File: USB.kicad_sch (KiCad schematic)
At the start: 31 parts, among them J5 USB_C_Receptacle, J6 USB_C_Receptacle, SW1 SW_DIP_x04, U10 TPS2552, U11 TPD4EUSB30, U12 TPD4EUSB30, U13 TPD4EUSB30, U14 TPD4EUSB30, U15 TS3USB221, U16 HD3SS3220, U17 TS3USB221

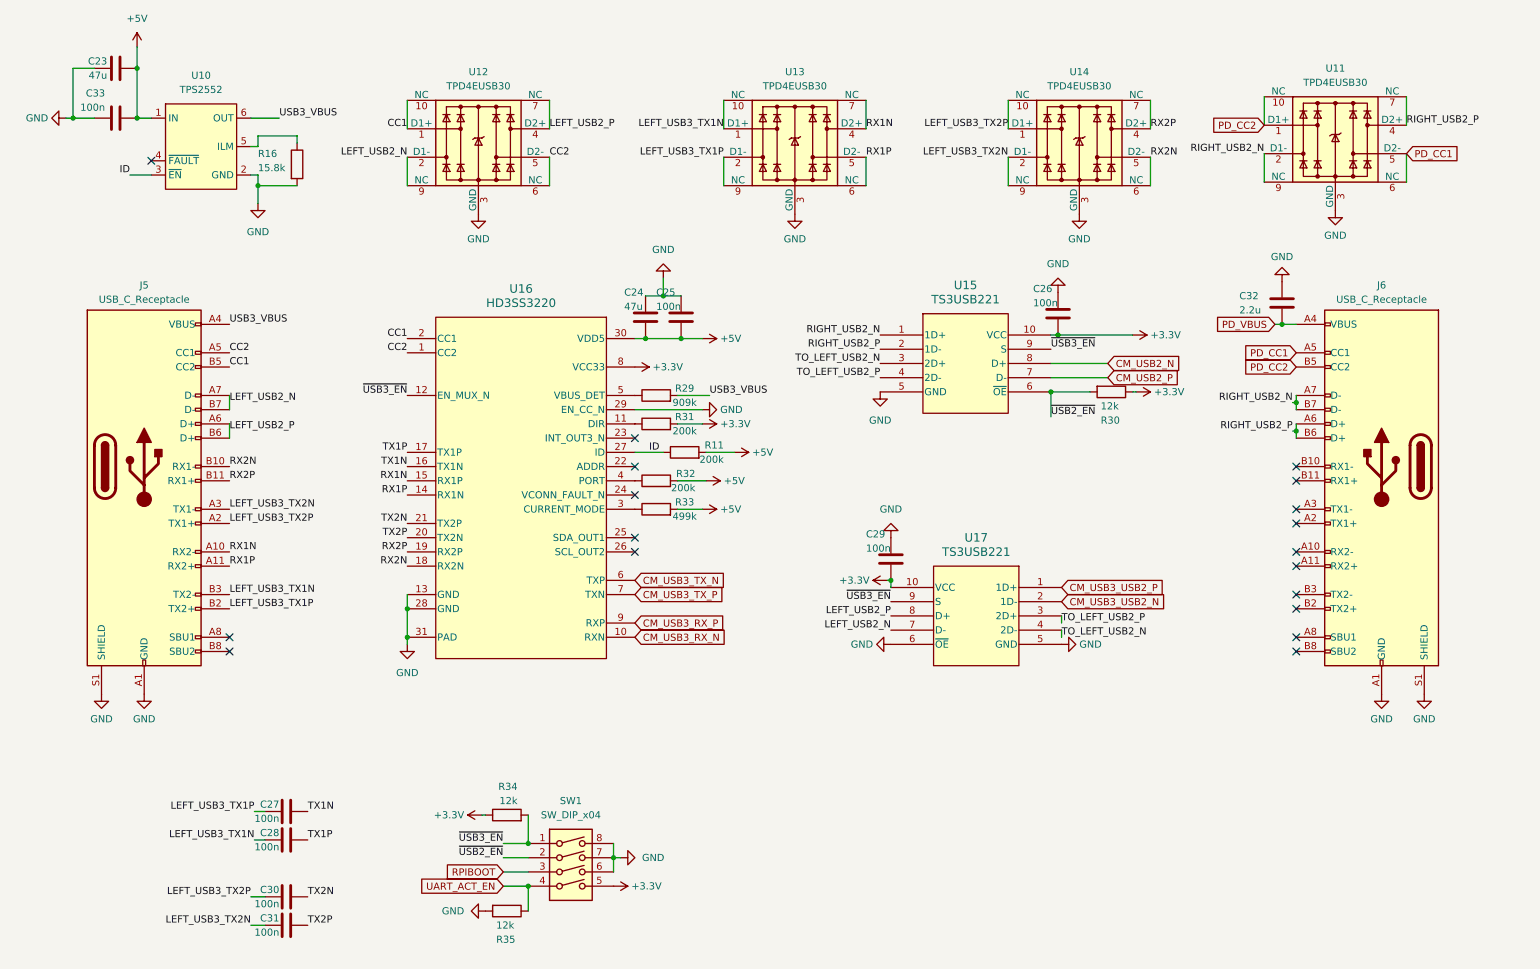
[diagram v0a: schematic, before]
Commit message: wip
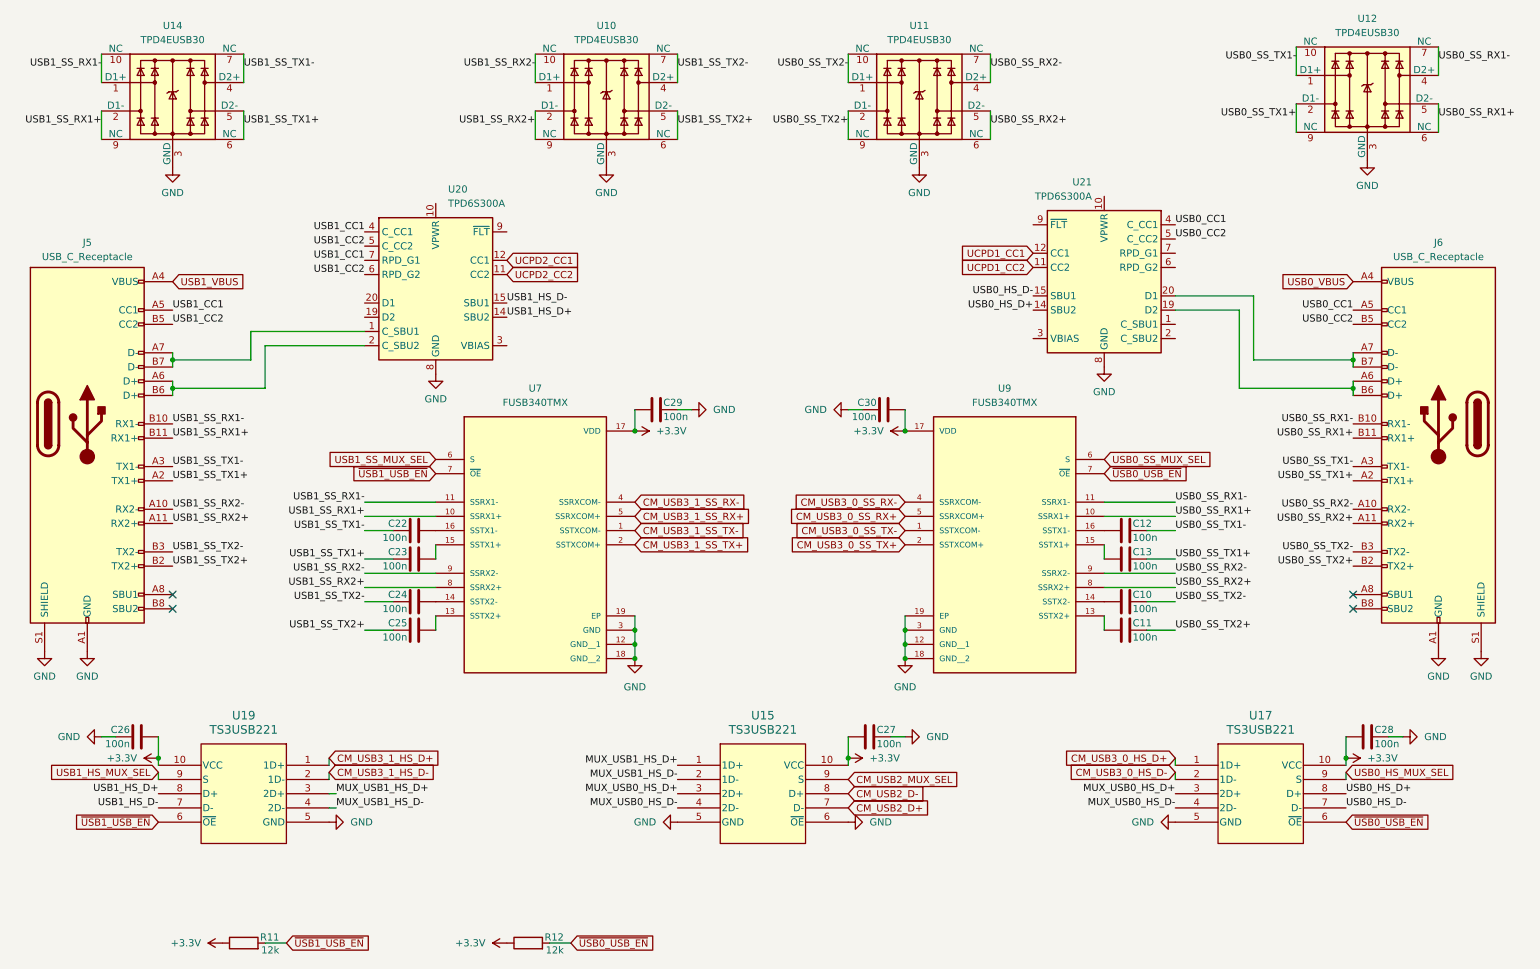
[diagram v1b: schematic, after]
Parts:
- removed C31, C33: 100n, Capacitor_SMD:C_0402_1005Metric, symbol Device:C
- removed C32: 2.2u, Capacitor_SMD:C_1206_3216Metric, symbol Device:C
- removed R16: 15.8k, Resistor_SMD:R_0402_1005Metric, symbol Device:R
- removed R29: 909k, Resistor_SMD:R_0402_1005Metric, symbol Device:R
- removed R30, R34, R35: 12k, Resistor_SMD:R_0402_1005Metric, symbol Device:R
- removed R31, R32: 200k, Resistor_SMD:R_0402_1005Metric, symbol Device:R
- removed R33: 499k, Resistor_SMD:R_0402_1005Metric, symbol Device:R
- removed SW1: SW_DIP_x04, PiCard:SW-SMD_8P-P1.27_EU-04KS, symbol Switch:SW_DIP_x04
- removed U10: TPS2552, Package_TO_SOT_SMD:SOT-23-6, symbol PiCard:TPS2552
- removed U13: TPD4EUSB30, Package_SON:USON-10_2.5x1.0mm_P0.5mm, symbol Power_Protection:TPD4EUSB30
- removed U16: HD3SS3220, PiCard:RNH0030A, symbol PiCard:HD3SS3220
- added C10, C11, C12, C13, C22: 100n, Capacitor_SMD:C_0402_1005Metric, symbol Device:C
- added R12: 12k, Resistor_SMD:R_0402_1005Metric, symbol Device:R
- added U10: TPD4EUSB30, Package_SON:USON-10_2.5x1.0mm_P0.5mm, symbol Power_Protection:TPD4EUSB30
- added U19: TS3USB221, PiCard:RSE10, symbol PiCard:TS3USB221
- added U20, U21: TPD6S300A, Package_DFN_QFN:WQFN-20-1EP_3x3mm_P0.4mm_EP1.7x1.7mm_ThermalVias, symbol Power_Protection:TPD6S300A
- added U7, U9: FUSB340TMX, PiCard:QFN-18-1EP_2x2.8mm_P0.4mm_EP1.05x1.85mm, symbol PiCard:FUSB340TMX
- C23, C24: value 47u -> 100n; footprint Capacitor_SMD:C_0805_2012Metric -> Capacitor_SMD:C_0402_1005Metric; LCSC C16780 -> C307331; MPN CL21A476MQYNNNE -> CL05B104KB54PNC
- R11: value 200k -> 12k; LCSC C25764 -> C25752; MPN 0402WGF2003TCE -> 0402WGF1202TCE
- U15, U17: footprint Package_DFN_QFN:Texas_UQFN-10_1.5x2mm_P0.5mm -> PiCard:RSE10; LCSC C130085 -> (none); MPN TS3USB221RSER -> (none); Manufacturer Texas Instruments -> (none)
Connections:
- net ID is gone; now on net +3.3V: R11.1
- net TX1N is gone; now on net +3.3V: C27.2
- net TX1P is gone; now on net +3.3V: C28.2
- net TX2N is gone; now on net +3.3V: C30.2
- net ~{USB2_EN} is gone; now on net GND: U15.6 (~{OE})
- net +3.3V: now also R12.1, U19.10 (VCC), U7.17 (VDD), U9.17 (VDD)
- net GND: now also C27.1, C28.1, C30.1, U10.3 (GND), U10.8 (GND), U19.5 (GND), U20.13 (GND), U20.16 (GND), U20.17 (GND), U20.18 (GND), U20.21 (GND), U20.8 (GND), U21.13 (GND), U21.16 (GND), U21.17 (GND), U21.18 (GND), U21.21 (GND), U21.8 (GND), U7.12 (GND__1), U7.18 (GND__2), U7.19 (EP), U7.3 (GND), U9.12 (GND__1), U9.18 (GND__2), U9.19 (EP), U9.3 (GND); no longer C23.1, C24.1, C25.1, U17.6 (~{OE})
- net USB0_SS_RX2-: now reaches J6.A10 (RX2-)
- net USB0_SS_RX2-: now also U11.4 (D2+), U11.7 (NC), U9.9 (SSRX2-)
- net USB0_SS_RX2+: now reaches J6.A11 (RX2+)
- net USB0_SS_RX2+: now also U11.5 (D2-), U11.6 (NC), U9.8 (SSRX2+)
- net USB0_SS_TX1+: now reaches J6.A2 (TX1+)
- net USB0_SS_TX1+: now also U12.2 (D1-), U12.9 (NC), C13.1
- net USB0_SS_TX1-: now reaches J6.A3 (TX1-)
- net USB0_SS_TX1-: now also U12.1 (D1+), U12.10 (NC), C12.1
- net USB0_SS_RX1-: now reaches J6.B10 (RX1-)
- net USB0_SS_RX1-: now also U12.4 (D2+), U12.7 (NC), U9.11 (SSRX1-)
- net USB0_SS_RX1+: now reaches J6.B11 (RX1+)
- net USB0_SS_RX1+: now also U12.5 (D2-), U12.6 (NC), U9.10 (SSRX1+)
- net USB0_SS_TX2+: now reaches J6.B2 (TX2+)
- net USB0_SS_TX2+: now also U11.2 (D1-), U11.9 (NC), C11.1
- net USB0_SS_TX2-: now reaches J6.B3 (TX2-)
- net USB0_SS_TX2-: now also U11.1 (D1+), U11.10 (NC), C10.1
- removed net +5V: C23.2, C24.2, C25.2, R11.2
- removed net CC1: J5.B5 (CC2), U12.1 (D1+), U12.10 (NC)
- removed net CC2: J5.A5 (CC1), U12.5 (D2-), U12.6 (NC)
- net CM_USB2_N renamed CM_USB2_D-
- net CM_USB2_P renamed CM_USB2_D+
- net CM_USB3_USB2_N renamed CM_USB3_0_HS_D-
- net CM_USB3_USB2_P renamed CM_USB3_0_HS_D+
- removed net LEFT_USB2_N: J5.A7 (D-), J5.B7 (D-), U12.2 (D1-), U12.9 (NC), U17.7 (D-)
- removed net LEFT_USB2_P: J5.A6 (D+), J5.B6 (D+), U12.4 (D2+), U12.7 (NC), U17.8 (D+)
- net LEFT_USB3_TX1N renamed USB1_SS_TX2-
- net USB1_SS_TX2-: now also C24.1, U10.4 (D2+), U10.7 (NC); no longer C28.1
- net LEFT_USB3_TX1P renamed USB1_SS_TX2+
- net USB1_SS_TX2+: now also C25.1, U10.5 (D2-), U10.6 (NC); no longer C27.1
- net LEFT_USB3_TX2N renamed USB1_SS_RX1+
- net USB1_SS_RX1+: now also J5.B11 (RX1+), U7.10 (SSRX1+); no longer J5.A3 (TX1-)
- net LEFT_USB3_TX2P renamed USB1_SS_RX1-
- net USB1_SS_RX1-: now also J5.B10 (RX1-), U7.11 (SSRX1-); no longer C30.1, J5.A2 (TX1+)
- removed net PD_CC1: J6.A5 (CC1), U11.5 (D2-), U11.6 (NC)
- removed net PD_CC2: J6.B5 (CC2), U11.1 (D1+), U11.10 (NC)
- net PD_VBUS renamed USB0_VBUS
- removed net RIGHT_USB2_N: J6.A7 (D-), J6.B7 (D-), U11.2 (D1-), U11.9 (NC), U15.1 (1D+)
- removed net RIGHT_USB2_P: J6.A6 (D+), J6.B6 (D+), U11.4 (D2+), U11.7 (NC), U15.2 (1D-)
- net RX1N renamed USB1_SS_RX2-
- net USB1_SS_RX2-: now also U10.1 (D1+), U10.10 (NC), U7.9 (SSRX2-)
- net RX1P renamed USB1_SS_RX2+
- net USB1_SS_RX2+: now also U10.2 (D1-), U10.9 (NC), U7.8 (SSRX2+)
- net RX2N renamed USB1_SS_TX1+
- net USB1_SS_TX1+: now also C23.1, J5.A2 (TX1+); no longer J5.B10 (RX1-)
- net RX2P renamed USB1_SS_TX1-
- net USB1_SS_TX1-: now also J5.A3 (TX1-), C22.1; no longer J5.B11 (RX1+)
- net TO_LEFT_USB2_N renamed MUX_USB0_HS_D+
- net MUX_USB0_HS_D+: now also U17.3 (2D+); no longer U17.4 (2D-)
- net TO_LEFT_USB2_P renamed MUX_USB0_HS_D-
- net MUX_USB0_HS_D-: now also U17.4 (2D-); no longer U17.3 (2D+)
- net USB3_VBUS renamed USB1_VBUS
- net ~{USB3_EN} renamed CM_USB2_MUX_SEL
- net CM_USB2_MUX_SEL: no longer U17.9 (S)
- new net: C10.2, U9.14 (SSTX2-)
- new net: C12.2, U9.16 (SSTX1-)
- new net: J6.A6 (D+), J6.B6 (D+), U21.19 (D2)
- new net: J6.A7 (D-), J6.B7 (D-), U21.20 (D1)
- new net: C25.2, U7.13 (SSTX2+)
- new net: C11.2, U9.13 (SSTX2+)
- new net: C13.2, U9.15 (SSTX1+)
- new net: C22.2, U7.16 (SSTX1-)
- new net: J5.A7 (D-), J5.B7 (D-), U20.1 (C_SBU1)
- new net: J5.A6 (D+), J5.B6 (D+), U20.2 (C_SBU2)
- new net: C23.2, U7.15 (SSTX1+)
- new net: C24.2, U7.14 (SSTX2-)
- new net CM_USB3_0_SS_RX+: U9.5 (SSRXCOM+)
- new net CM_USB3_0_SS_RX-: U9.4 (SSRXCOM-)
- new net CM_USB3_0_SS_TX+: U9.2 (SSTXCOM+)
- new net CM_USB3_0_SS_TX-: U9.1 (SSTXCOM-)
- new net CM_USB3_1_HS_D+: U19.1 (1D+)
- new net CM_USB3_1_HS_D-: U19.2 (1D-)
- new net CM_USB3_1_SS_RX+: U7.5 (SSRXCOM+)
- new net CM_USB3_1_SS_RX-: U7.4 (SSRXCOM-)
- new net CM_USB3_1_SS_TX+: U7.2 (SSTXCOM+)
- new net CM_USB3_1_SS_TX-: U7.1 (SSTXCOM-)
- new net MUX_USB1_HS_D+: U15.1 (1D+), U19.3 (2D+)
- new net MUX_USB1_HS_D-: U15.2 (1D-), U19.4 (2D-)
- new net UCPD1_CC1: U21.12 (CC1)
- new net UCPD1_CC2: U21.11 (CC2)
- new net UCPD2_CC1: U20.12 (CC1)
- new net UCPD2_CC2: U20.11 (CC2)
- new net USB0_CC1: J6.A5 (CC1), U21.4 (C_CC1)
- new net USB0_CC2: J6.B5 (CC2), U21.5 (C_CC2)
- new net USB0_HS_D+: U17.8 (D+), U21.14 (SBU2)
- new net USB0_HS_D-: U17.7 (D-), U21.15 (SBU1)
- new net USB0_HS_MUX_SEL: U17.9 (S)
- new net USB0_SS_MUX_SEL: U9.6 (S)
- new net USB1_CC1: J5.A5 (CC1), U20.4 (C_CC1), U20.7 (RPD_G1)
- new net USB1_CC2: J5.B5 (CC2), U20.5 (C_CC2), U20.6 (RPD_G2)
- new net USB1_HS_D+: U19.8 (D+), U20.14 (SBU2)
- new net USB1_HS_D-: U19.7 (D-), U20.15 (SBU1)
- new net USB1_HS_MUX_SEL: U19.9 (S)
- new net USB1_SS_MUX_SEL: U7.6 (S)
- new net ~{USB0_USB_EN}: R12.2, U17.6 (~{OE}), U9.7 (~{OE})
- new net ~{USB1_USB_EN}: R11.2, U19.6 (~{OE}), U7.7 (~{OE})
- no-connect marks 18 -> 4
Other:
- moved on the sheet: J5, J6, U14
